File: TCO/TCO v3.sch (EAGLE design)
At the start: 19 parts

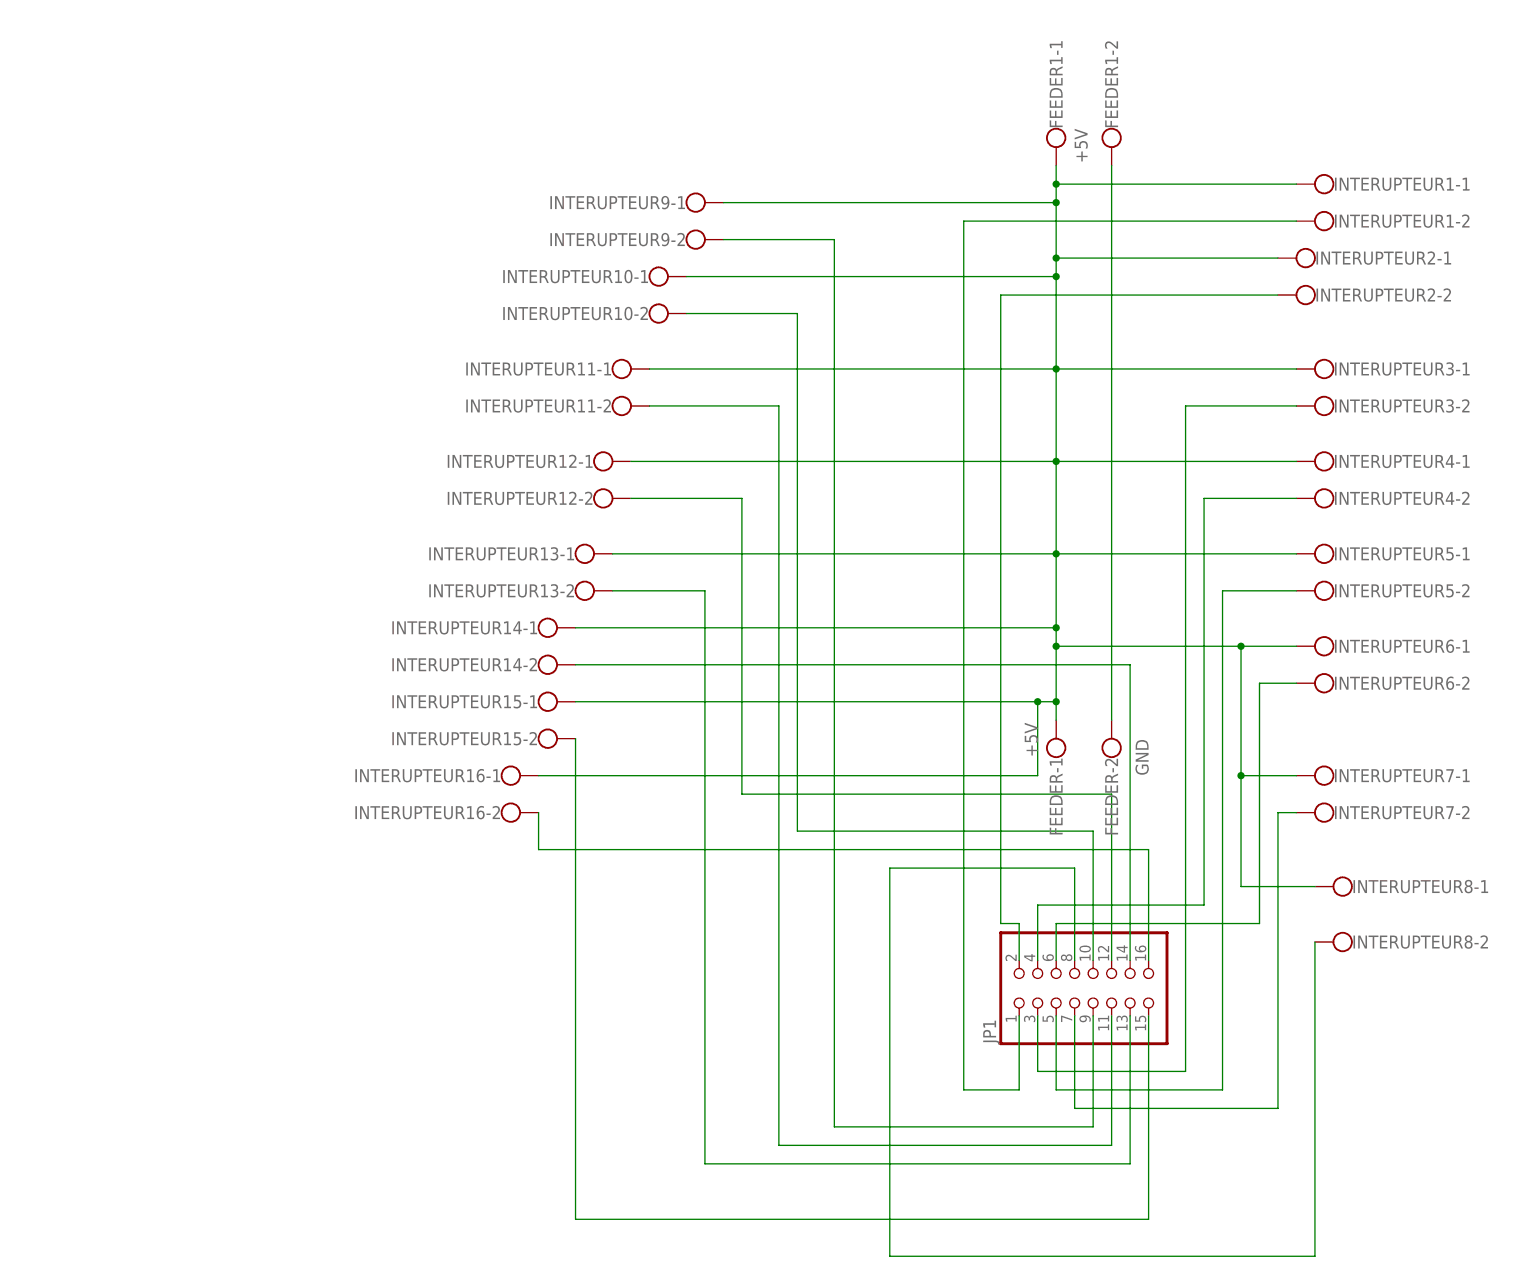
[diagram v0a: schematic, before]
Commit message: update
optimisation de mmontage
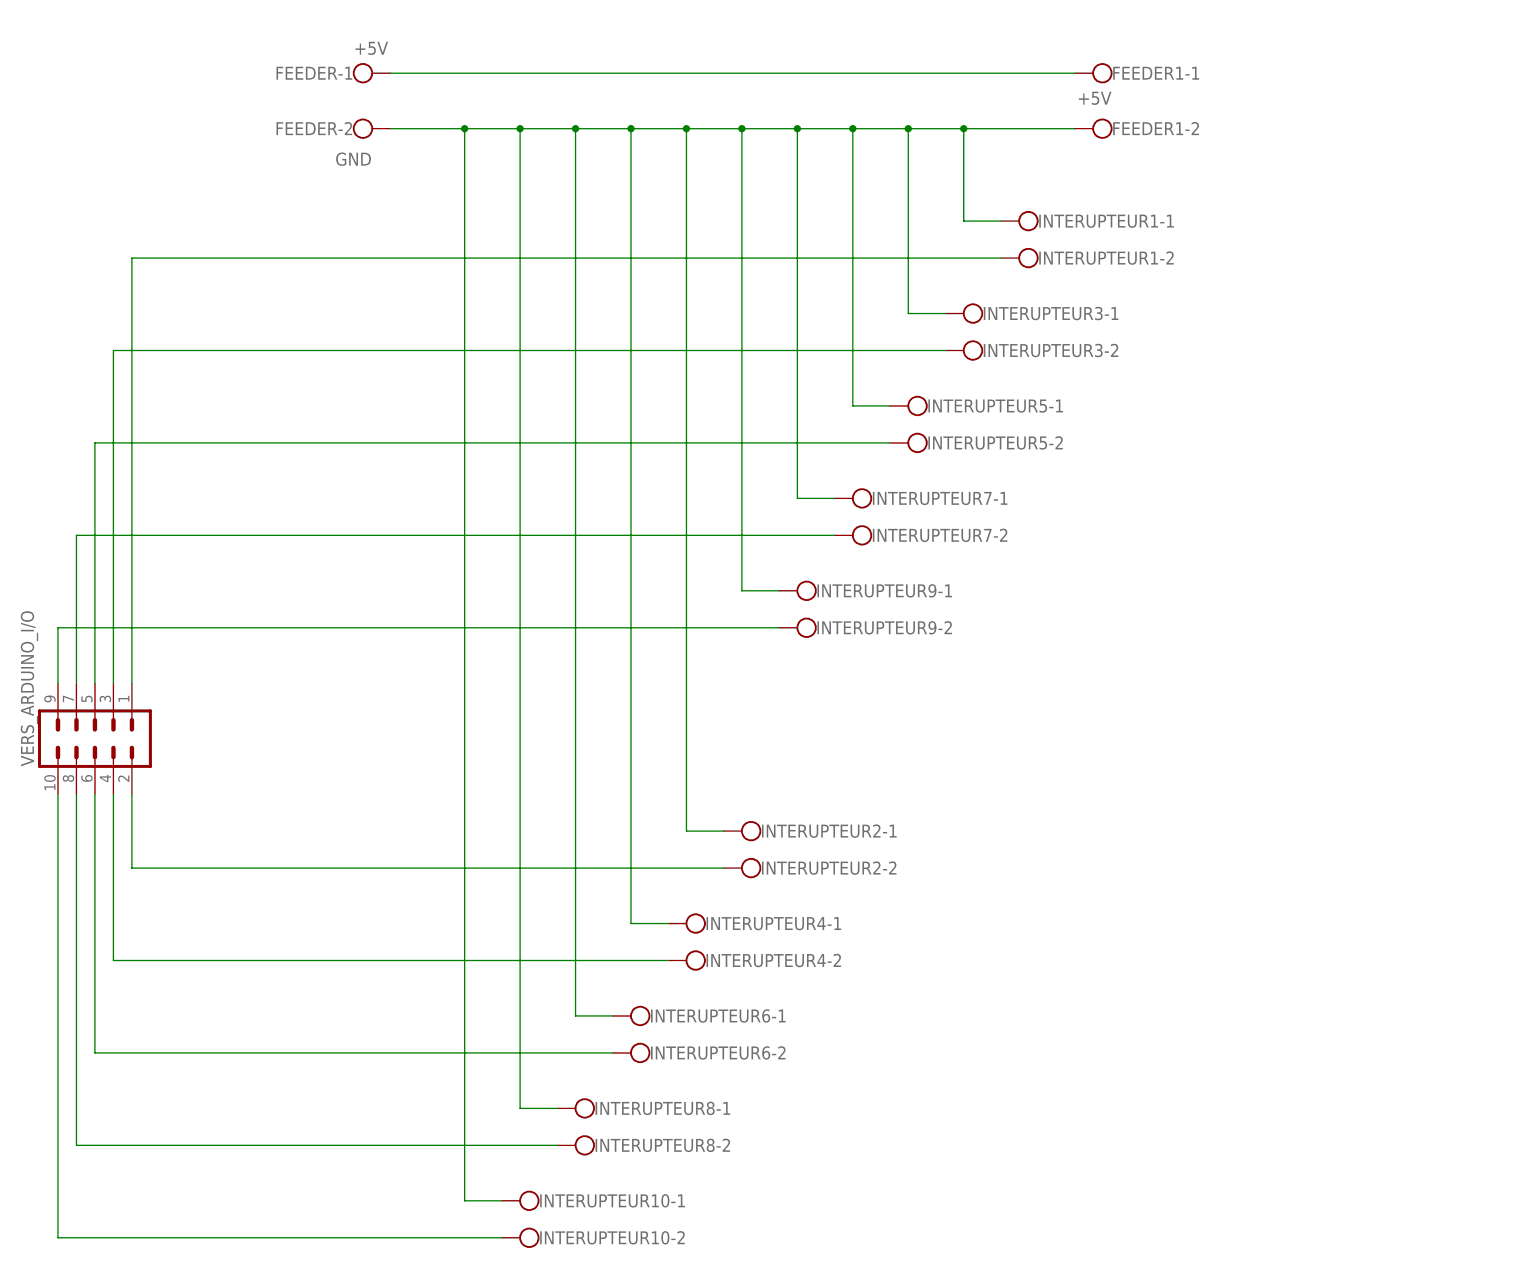
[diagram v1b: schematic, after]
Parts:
- removed INTERUPTEUR11, INTERUPTEUR12, INTERUPTEUR13, INTERUPTEUR14, INTERUPTEUR15, INTERUPTEUR16: (no value), con-wago-500:W237-102
- removed JP1: (no value), pinhead:PINHD-2X8
- added VERS_ARDUINO_I/O: (no value), con-lstb:MA05-2
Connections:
- removed net N$12: INTERUPTEUR10-2.KL, JP1.10
- removed net N$13: INTERUPTEUR11-2.KL, JP1.11
- removed net N$14: INTERUPTEUR12-2.KL, JP1.12
- removed net N$15: INTERUPTEUR13-2.KL, JP1.13
- removed net N$16: INTERUPTEUR14-2.KL, JP1.14
- removed net N$17: INTERUPTEUR15-2.KL, JP1.15
- removed net N$18: INTERUPTEUR16-2.KL, JP1.16
- new net N$26: FEEDER-2.KL, FEEDER1-2.KL, INTERUPTEUR1-1.KL, INTERUPTEUR10-1.KL, INTERUPTEUR2-1.KL, INTERUPTEUR3-1.KL, INTERUPTEUR4-1.KL, INTERUPTEUR5-1.KL, INTERUPTEUR6-1.KL, INTERUPTEUR7-1.KL, INTERUPTEUR8-1.KL, INTERUPTEUR9-1.KL
- net N$1: no longer INTERUPTEUR1-1.KL, INTERUPTEUR10-1.KL, INTERUPTEUR11-1.KL, INTERUPTEUR12-1.KL, INTERUPTEUR13-1.KL, INTERUPTEUR14-1.KL, INTERUPTEUR15-1.KL, INTERUPTEUR16-1.KL, INTERUPTEUR2-1.KL, INTERUPTEUR3-1.KL, INTERUPTEUR4-1.KL, INTERUPTEUR5-1.KL, INTERUPTEUR6-1.KL, INTERUPTEUR7-1.KL, INTERUPTEUR8-1.KL, INTERUPTEUR9-1.KL
- net N$10: now also VERS_ARDUINO_I/O.8; no longer JP1.8
- net N$11: now also INTERUPTEUR10-2.KL, VERS_ARDUINO_I/O.10; no longer INTERUPTEUR9-2.KL, JP1.9
- net N$2: now also INTERUPTEUR1-2.KL, VERS_ARDUINO_I/O.1; no longer FEEDER-2.KL, FEEDER1-2.KL
- net N$3: now also INTERUPTEUR3-2.KL, VERS_ARDUINO_I/O.3; no longer INTERUPTEUR1-2.KL, JP1.1
- net N$4: now also INTERUPTEUR5-2.KL, VERS_ARDUINO_I/O.5; no longer INTERUPTEUR2-2.KL, JP1.2
- net N$5: now also INTERUPTEUR7-2.KL, VERS_ARDUINO_I/O.7; no longer INTERUPTEUR3-2.KL, JP1.3
- net N$6: now also INTERUPTEUR9-2.KL, VERS_ARDUINO_I/O.9; no longer INTERUPTEUR4-2.KL, JP1.4
- net N$7: now also INTERUPTEUR2-2.KL, VERS_ARDUINO_I/O.2; no longer INTERUPTEUR5-2.KL, JP1.5
- net N$8: now also INTERUPTEUR4-2.KL, VERS_ARDUINO_I/O.4; no longer INTERUPTEUR6-2.KL, JP1.6
- net N$9: now also INTERUPTEUR6-2.KL, VERS_ARDUINO_I/O.6; no longer INTERUPTEUR7-2.KL, JP1.7
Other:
- moved on the sheet: FEEDER-1, FEEDER-2, FEEDER1-1, FEEDER1-2, INTERUPTEUR1-1, INTERUPTEUR1-2, INTERUPTEUR10-1, INTERUPTEUR10-2, INTERUPTEUR2-1, INTERUPTEUR2-2, INTERUPTEUR3-1, INTERUPTEUR3-2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
